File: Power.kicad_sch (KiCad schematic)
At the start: 2 parts

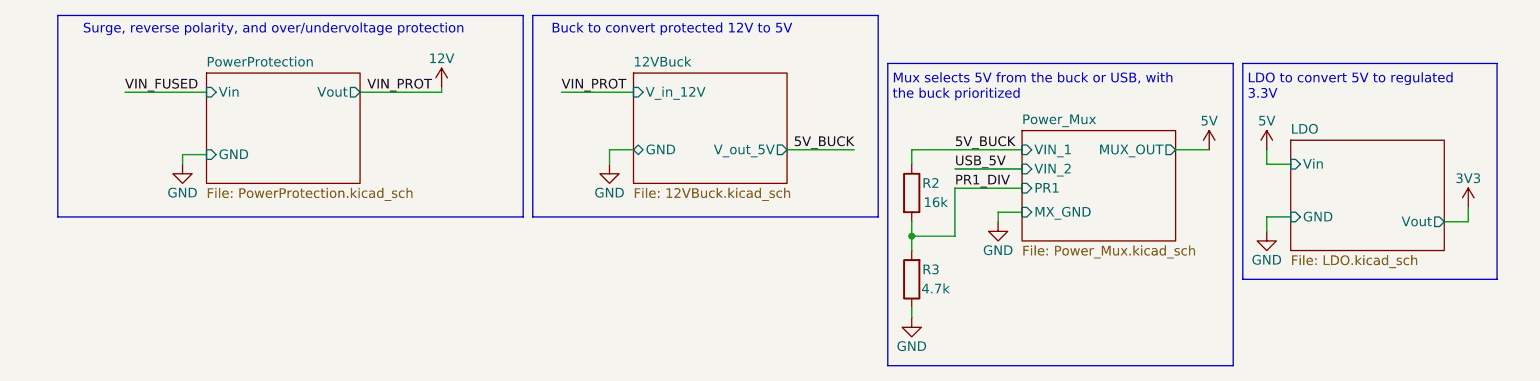
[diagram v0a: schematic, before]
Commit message: saving
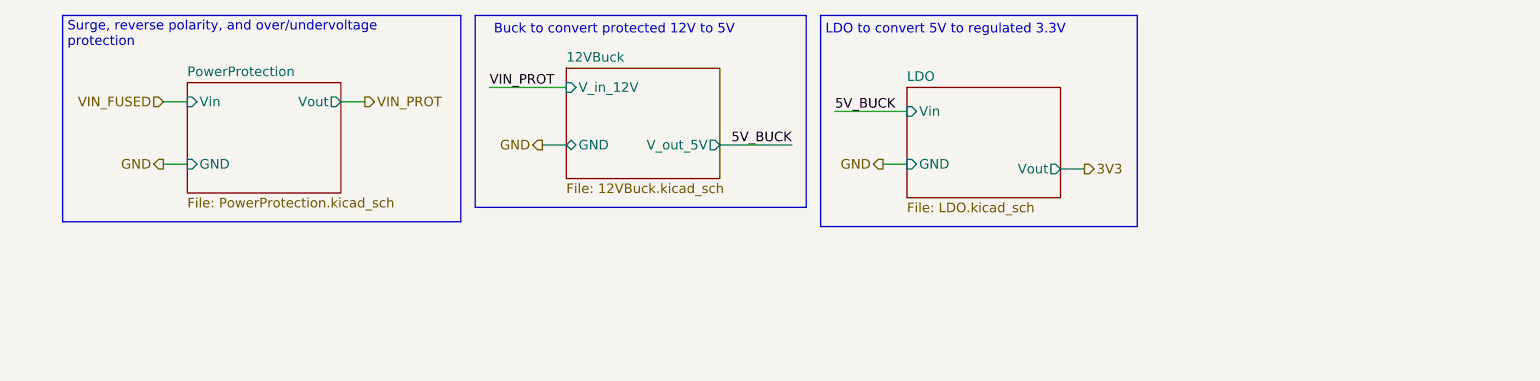
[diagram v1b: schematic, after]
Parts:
- removed R2: 16k, Package_DIP:DIP-8_W7.62mm, symbol Device:R
- removed R3: 4.7k, Package_DIP:DIP-8_W7.62mm, symbol Device:R
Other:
- removed sheet Power_Mux
- note removed: "Mux selects 5V from the buck or USB, with the buck prioritized"
